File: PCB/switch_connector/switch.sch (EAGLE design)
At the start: 7 parts

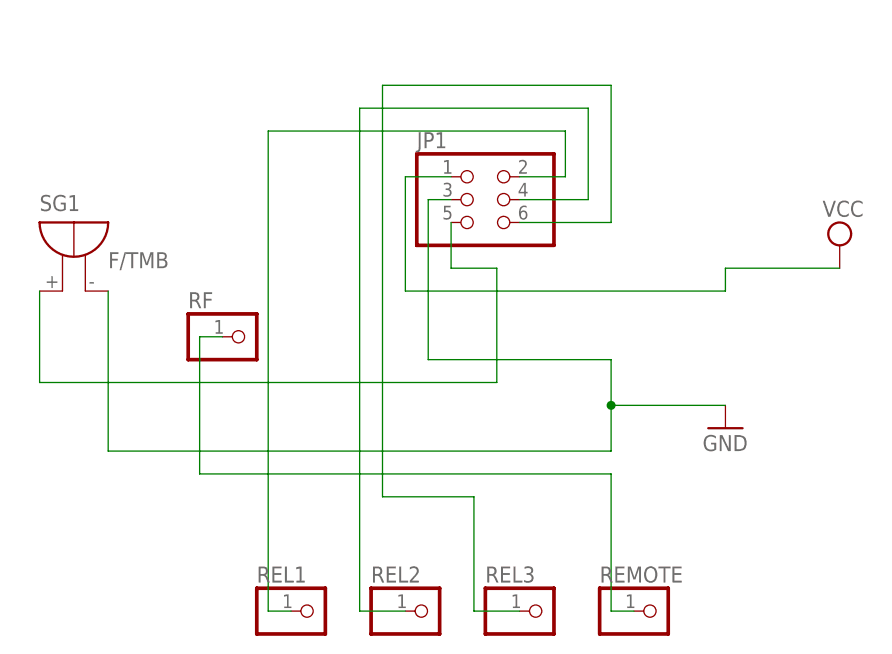
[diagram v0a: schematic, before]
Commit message: all files
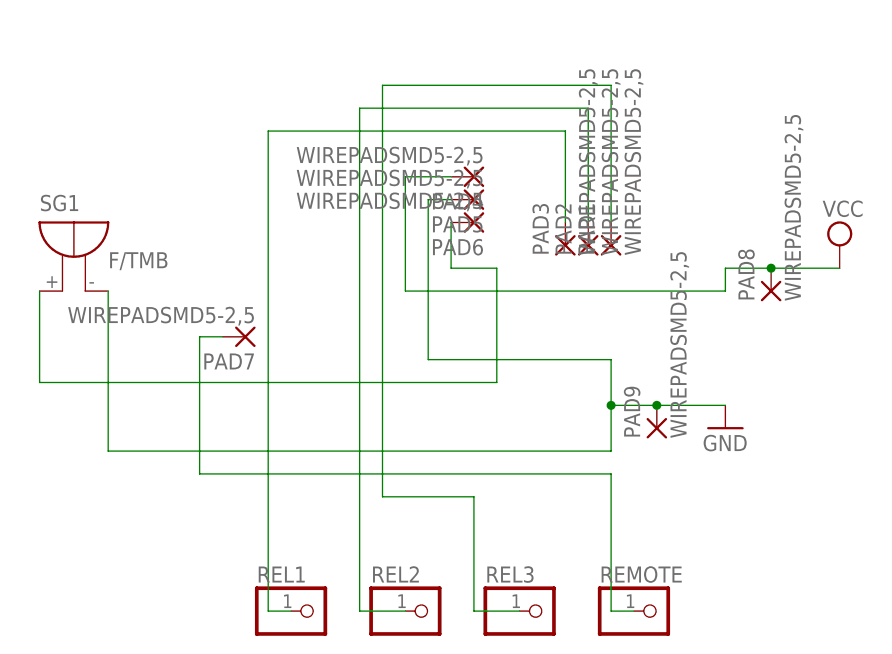
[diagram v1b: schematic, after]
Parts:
- removed JP1: (no value), pinhead:PINHD-2X3
- removed RF: (no value), pinhead:PINHD-1X1
- added PAD1, PAD2, PAD3, PAD4, PAD5, PAD6, PAD7, PAD8, PAD9: WIREPADSMD5-2,5, wirepad:WIREPADSMD5-2,5
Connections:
- net GND: now also PAD5.P, PAD9.P; no longer JP1.3
- net N$1: now also PAD3.P; no longer JP1.2
- net N$10: now also PAD6.P; no longer JP1.5
- net N$2: now also PAD2.P; no longer JP1.4
- net N$3: now also PAD1.P; no longer JP1.6
- net N$7: now also PAD7.P; no longer RF.1
- net VCC: now also PAD4.P, PAD8.P; no longer JP1.1
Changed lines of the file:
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@@
 <part name="REL3" library="pinhead" library_urn="urn:adsk.eagle:library:325" deviceset="PINHD-1X1" device="" package3d_urn="urn:adsk.eagle:package:22485/2"/>
 <part name="REMOTE" library="pinhead" library_urn="urn:adsk.eagle:library:325" deviceset="PINHD-1X1" device="" package3d_urn="urn:adsk.eagle:package:22485/2"/>
-<part name="RF" library="pinhead" library_urn="urn:adsk.eagle:library:325" deviceset="PINHD-1X1" device="" package3d_urn="urn:adsk.eagle:package:22485/2"/>
 <part name="SG1" library="buzzer" library_urn="urn:adsk.eagle:library:113" deviceset="F/TMB" device="" package3d_urn="urn:adsk.eagle:package:5260/1"/>
-<part name="JP1" library="pinhead" library_urn="urn:adsk.eagle:library:325" deviceset="PINHD-2X3" device="" package3d_urn="urn:adsk.eagle:package:22462/2"/>
+<part name="PAD1" library="wirepad" library_urn="urn:adsk.eagle:library:412" deviceset="WIREPAD" device="SMD5-2,5" package3d_urn="urn:adsk.eagle:package:30845/1"/>
+<part name="PAD2" library="wirepad" library_urn="urn:adsk.eagle:library:412" deviceset="WIREPAD" device="SMD5-2,5" package3d_urn="urn:adsk.eagle:package:30845/1"/>
+<part name="PAD3" library="wirepad" library_urn="urn:adsk.eagle:library:412" deviceset="WIREPAD" device="SMD5-2,5" package3d_urn="urn:adsk.eagle:package:30845/1"/>
+<part name="PAD4" library="wirepad" library_urn="urn:adsk.eagle:library:412" deviceset="WIREPAD" device="SMD5-2,5" package3d_urn="urn:adsk.eagle:package:30845/1"/>
+<part name="PAD5" library="wirepad" library_urn="urn:adsk.eagle:library:412" deviceset="WIREPAD" device="SMD5-2,5" package3d_urn="urn:adsk.eagle:package:30845/1"/>
+<part name="PAD6" library="wirepad" library_urn="urn:adsk.eagle:library:412" deviceset="WIREPAD" device="SMD5-2,5" package3d_urn="urn:adsk.eagle:package:30845/1"/>
+<part name="PAD7" library="wirepad" library_urn="urn:adsk.eagle:library:412" deviceset="WIREPAD" device="SMD5-2,5" package3d_urn="urn:adsk.eagle:package:30845/1"/>
+<part name="PAD8" library="wirepad" library_urn="urn:adsk.eagle:library:412" deviceset="WIREPAD" device="SMD5-2,5" package3d_urn="urn:adsk.eagle:package:30845/1"/>
+<part name="PAD9" library="wirepad" library_urn="urn:adsk.eagle:library:412" deviceset="WIREPAD" device="SMD5-2,5" package3d_urn="urn:adsk.eagle:package:30845/1"/>
 </parts>
 <sheets>
@@
 <instance part="REL3" gate="G$1" x="66.04" y="12.7"/>
 <instance part="REMOTE" gate="G$1" x="78.74" y="12.7"/>
-<instance part="RF" gate="G$1" x="33.02" y="43.18"/>
 <instance part="SG1" gate="1" x="12.7" y="50.8"/>
-<instance part="JP1" gate="A" x="58.42" y="58.42"/>
+<instance part="PAD1" gate="G$1" x="73.66" y="53.34" rot="R90"/>
+<instance part="PAD2" gate="G$1" x="71.12" y="53.34" rot="R90"/>
+<instance part="PAD3" gate="G$1" x="68.58" y="53.34" rot="R90"/>
+<instance part="PAD4" gate="G$1" x="58.42" y="60.96" rot="R180"/>
+<instance part="PAD5" gate="G$1" x="58.42" y="58.42" rot="R180"/>
+<instance part="PAD6" gate="G$1" x="58.42" y="55.88" rot="R180"/>
+<instance part="PAD7" gate="G$1" x="33.02" y="43.18" rot="R180"/>
+<instance part="PAD8" gate="G$1" x="91.44" y="48.26" rot="R90"/>
+<instance part="PAD9" gate="G$1" x="78.74" y="33.02" rot="R90"/>
 </instances>
 <busses>
@@
 <pinref part="REL1" gate="G$1" pin="1"/>
 <wire x1="35.56" y1="12.7" x2="38.1" y2="12.7" width="0.1524" layer="91"/>
-<pinref part="JP1" gate="A" pin="2"/>
-<wire x1="63.5" y1="60.96" x2="68.58" y2="60.96" width="0.1524" layer="91"/>
-<wire x1="68.58" y1="60.96" x2="68.58" y2="66.04" width="0.1524" layer="91"/>
+<wire x1="68.58" y1="66.04" x2="68.58" y2="55.88" width="0.1524" layer="91"/>
+<pinref part="PAD3" gate="G$1" pin="P"/>
 </segment>
 </net>
@@
 <pinref part="REL2" gate="G$1" pin="1"/>
 <wire x1="45.72" y1="12.7" x2="50.8" y2="12.7" width="0.1524" layer="91"/>
-<pinref part="JP1" gate="A" pin="4"/>
-<wire x1="63.5" y1="58.42" x2="71.12" y2="58.42" width="0.1524" layer="91"/>
-<wire x1="71.12" y1="58.42" x2="71.12" y2="68.58" width="0.1524" layer="91"/>
+<wire x1="71.12" y1="55.88" x2="71.12" y2="68.58" width="0.1524" layer="91"/>
 <wire x1="71.12" y1="68.58" x2="45.72" y2="68.58" width="0.1524" layer="91"/>
+<pinref part="PAD2" gate="G$1" pin="P"/>
 </segment>
 </net>
@@
 <pinref part="REL3" gate="G$1" pin="1"/>
 <wire x1="58.42" y1="12.7" x2="63.5" y2="12.7" width="0.1524" layer="91"/>
-<pinref part="JP1" gate="A" pin="6"/>
-<wire x1="63.5" y1="55.88" x2="73.66" y2="55.88" width="0.1524" layer="91"/>
 <wire x1="73.66" y1="55.88" x2="73.66" y2="71.12" width="0.1524" layer="91"/>
 <wire x1="73.66" y1="71.12" x2="48.26" y2="71.12" width="0.1524" layer="91"/>
+<pinref part="PAD1" gate="G$1" pin="P"/>
 </segment>
 </net>
@@
 <segment>
 <pinref part="SUPPLY1" gate="G$1" pin="VCC"/>
-<wire x1="86.36" y1="50.8" x2="99.06" y2="50.8" width="0.1524" layer="91"/>
+<wire x1="86.36" y1="50.8" x2="91.44" y2="50.8" width="0.1524" layer="91"/>
+<wire x1="91.44" y1="50.8" x2="99.06" y2="50.8" width="0.1524" layer="91"/>
 <wire x1="86.36" y1="50.8" x2="86.36" y2="48.26" width="0.1524" layer="91"/>
 <wire x1="86.36" y1="48.26" x2="50.8" y2="48.26" width="0.1524" layer="91"/>
-<pinref part="JP1" gate="A" pin="1"/>
 <wire x1="55.88" y1="60.96" x2="50.8" y2="60.96" width="0.1524" layer="91"/>
 <wire x1="50.8" y1="60.96" x2="50.8" y2="48.26" width="0.1524" layer="91"/>
+<pinref part="PAD4" gate="G$1" pin="P"/>
+<pinref part="PAD8" gate="G$1" pin="P"/>
+<junction x="91.44" y="50.8"/>
 </segment>
 </net>
@@
 <segment>
 <pinref part="GND1" gate="1" pin="GND"/>
-<wire x1="73.66" y1="35.56" x2="86.36" y2="35.56" width="0.1524" layer="91"/>
+<wire x1="73.66" y1="35.56" x2="78.74" y2="35.56" width="0.1524" layer="91"/>
+<wire x1="78.74" y1="35.56" x2="86.36" y2="35.56" width="0.1524" layer="91"/>
 <wire x1="17.78" y1="48.26" x2="17.78" y2="30.48" width="0.1524" layer="91"/>
 <wire x1="17.78" y1="30.48" x2="73.66" y2="30.48" width="0.1524" layer="91"/>
@@
 <junction x="73.66" y="35.56"/>
 <pinref part="SG1" gate="1" pin="-"/>
-<pinref part="JP1" gate="A" pin="3"/>
 <wire x1="55.88" y1="58.42" x2="53.34" y2="58.42" width="0.1524" layer="91"/>
 <wire x1="53.34" y1="58.42" x2="53.34" y2="40.64" width="0.1524" layer="91"/>
 <wire x1="53.34" y1="40.64" x2="73.66" y2="40.64" width="0.1524" layer="91"/>
 <wire x1="73.66" y1="40.64" x2="73.66" y2="35.56" width="0.1524" layer="91"/>
+<pinref part="PAD5" gate="G$1" pin="P"/>
+<pinref part="PAD9" gate="G$1" pin="P"/>
+<junction x="78.74" y="35.56"/>
 </segment>
 </net>
@@
 <pinref part="REMOTE" gate="G$1" pin="1"/>
 <wire x1="73.66" y1="12.7" x2="76.2" y2="12.7" width="0.1524" layer="91"/>
-<pinref part="RF" gate="G$1" pin="1"/>
 <wire x1="27.94" y1="43.18" x2="30.48" y2="43.18" width="0.1524" layer="91"/>
+<pinref part="PAD7" gate="G$1" pin="P"/>
 </segment>
 </net>
@@
 <pinref part="SG1" gate="1" pin="+"/>
 <wire x1="60.96" y1="38.1" x2="60.96" y2="50.8" width="0.1524" layer="91"/>
-<pinref part="JP1" gate="A" pin="5"/>
 <wire x1="55.88" y1="55.88" x2="55.88" y2="50.8" width="0.1524" layer="91"/>
 <wire x1="55.88" y1="50.8" x2="60.96" y2="50.8" width="0.1524" layer="91"/>
+<pinref part="PAD6" gate="G$1" pin="P"/>
 </segment>
 </net>
